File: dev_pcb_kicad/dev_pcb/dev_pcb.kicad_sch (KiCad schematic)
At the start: 11 parts, among them U2 XIAO-ESP32-S3-DIP

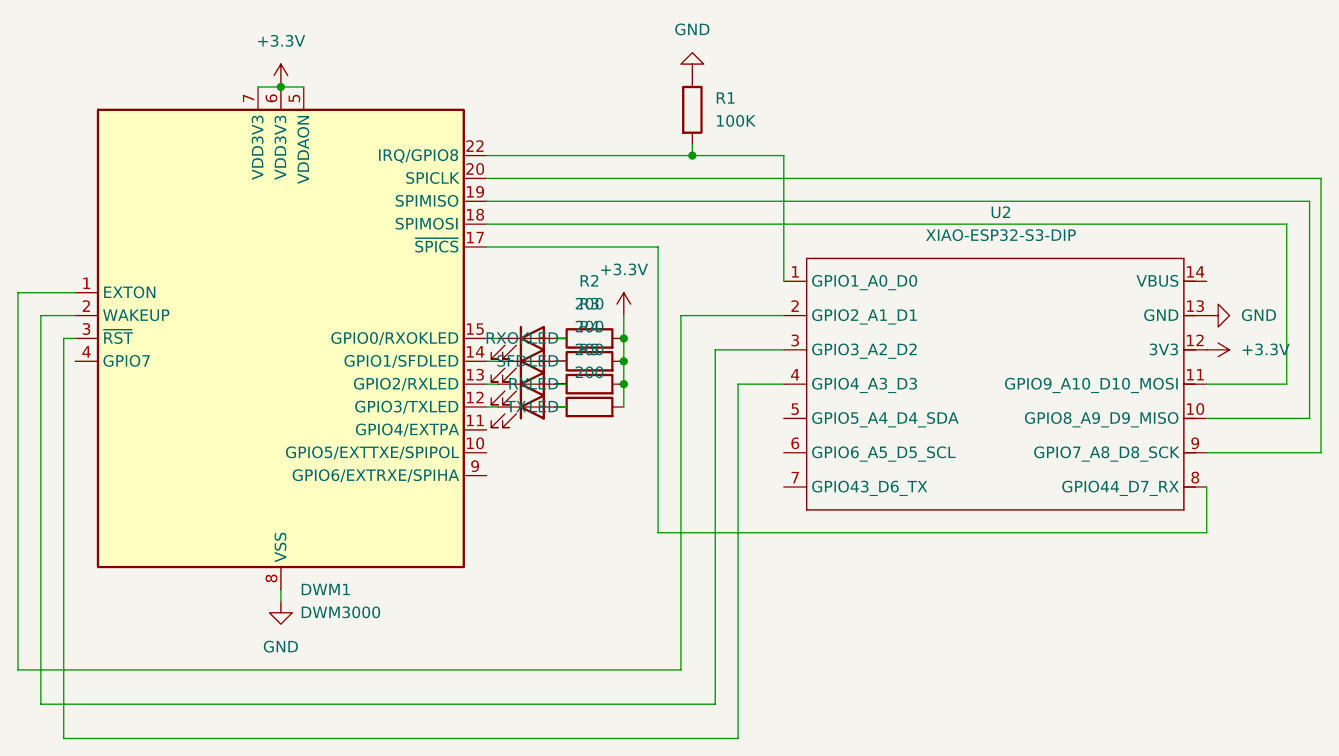
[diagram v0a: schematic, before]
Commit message: probe points
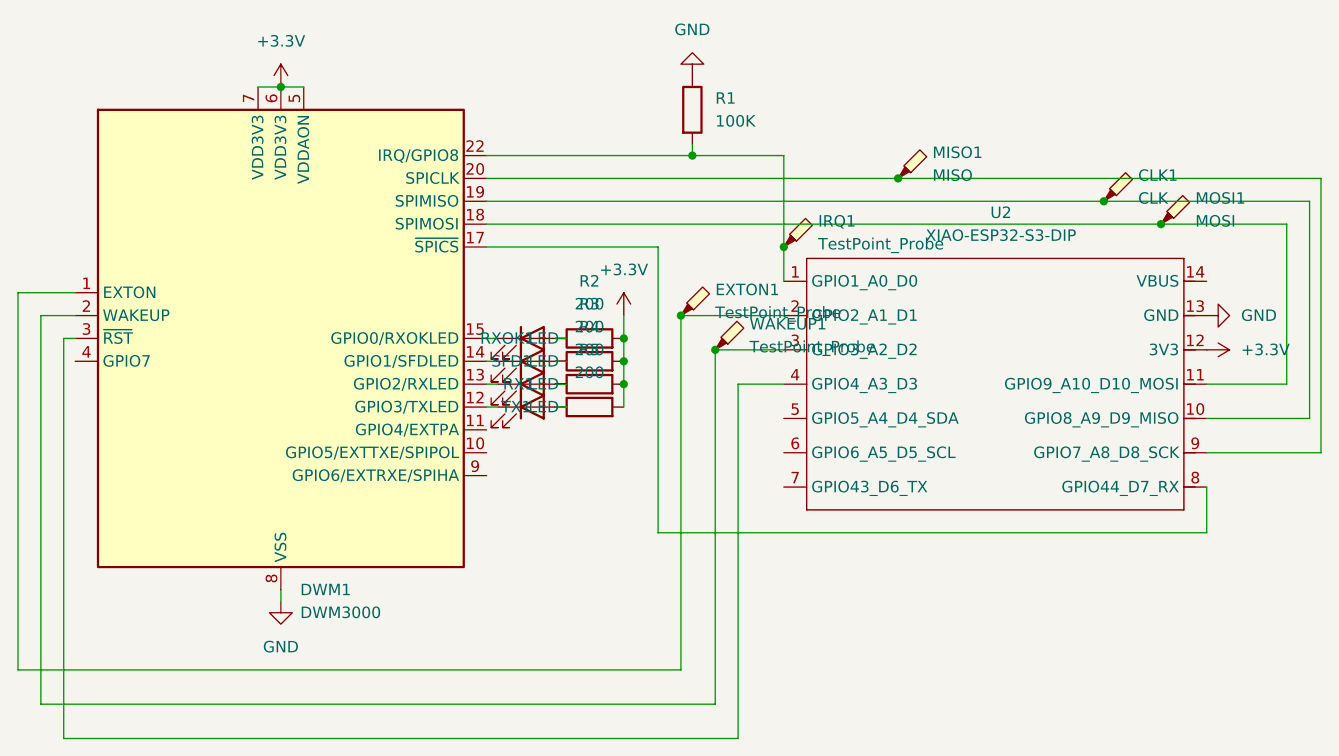
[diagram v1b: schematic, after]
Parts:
- added CLK1: CLK, TestPoint:TestPoint_Pad_D1.0mm, symbol Connector:TestPoint_Probe
- added EXTON1, IRQ1, WAKEUP1: TestPoint_Probe, TestPoint:TestPoint_Pad_D1.0mm, symbol Connector:TestPoint_Probe
- added MISO1: MISO, TestPoint:TestPoint_Pad_D1.0mm, symbol Connector:TestPoint_Probe
- added MOSI1: MOSI, TestPoint:TestPoint_Pad_D1.0mm, symbol Connector:TestPoint_Probe
- renumbered RX to RX1, RXOK to RXOK1, SFD to SFD1, TX to TX1
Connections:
- net at DWM1.1 (EXTON), U2.2 (GPIO2_A1_D1): now also EXTON1.1
- net at DWM1.18 (SPIMOSI), U2.11 (GPIO9_A10_D10_MOSI): now also MOSI1.1
- net at DWM1.19 (SPIMISO), U2.10 (GPIO8_A9_D9_MISO): now also CLK1.1
- net at DWM1.2 (WAKEUP), U2.3 (GPIO3_A2_D2): now also WAKEUP1.1
- net at DWM1.20 (SPICLK), U2.9 (GPIO7_A8_D8_SCK): now also MISO1.1
- net at DWM1.22 (IRQ/GPIO8), R1.2, U2.1 (GPIO1_A0_D0): now also IRQ1.1
